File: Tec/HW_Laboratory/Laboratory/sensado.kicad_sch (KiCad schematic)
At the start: 21 parts, among them U5 INA3221, U6 INA3221, U7 LM75B

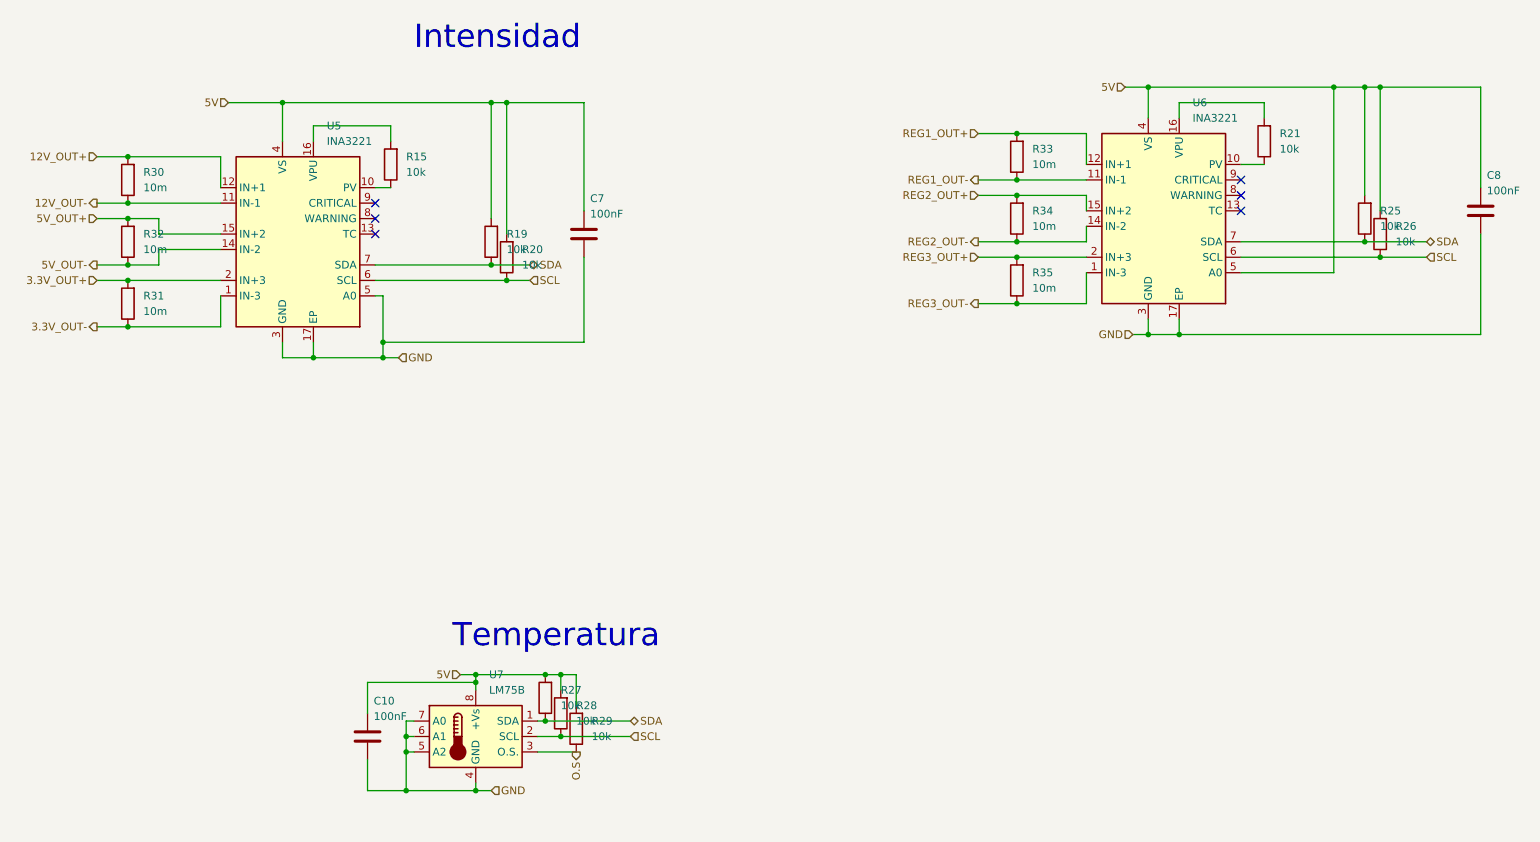
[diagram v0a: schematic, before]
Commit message: Laboratory v2.0:Update the PCB and the Software
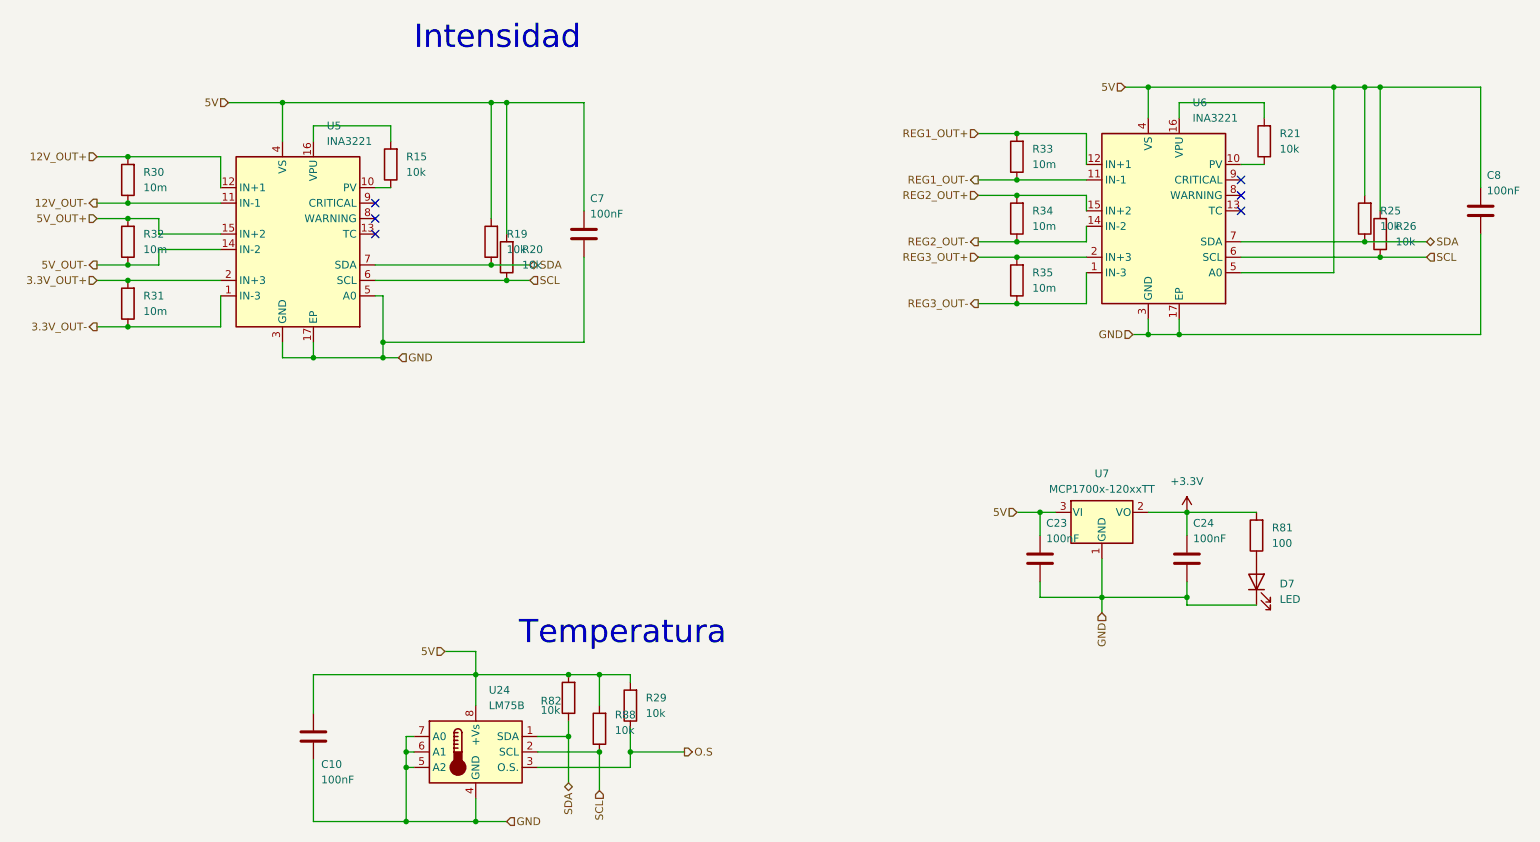
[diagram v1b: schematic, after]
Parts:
- removed R27, R28: 10k, Resistor_SMD:R_0603_1608Metric, symbol Device:R
- removed U7: LM75B, Package_SO:SOIC-8_3.9x4.9mm_P1.27mm, symbol Sensor_Temperature:LM75B
- added C23, C24: 100nF, Capacitor_SMD:C_0603_1608Metric, symbol Device:C
- added D7: LED, LED_SMD:LED_0603_1608Metric, symbol Device:LED
- added R81: 100, Resistor_SMD:R_0603_1608Metric, symbol Device:R
- added R82, R88: 10k, Resistor_SMD:R_0603_1608Metric, symbol Device:R
- added U24: LM75B, Package_SO:SOIC-8_3.9x4.9mm_P1.27mm, symbol Sensor_Temperature:LM75B
- added U7: MCP1700x-120xxTT, Package_TO_SOT_SMD:SOT-23, symbol Regulator_Linear:MCP1700x-120xxTT
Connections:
- net 5V: now also C23.1, R82.2, R88.2, U24.8 (+Vs), U7.3 (VI)
- net GND: now also C23.2, C24.2, D7.1 (K), U24.4 (GND), U24.5 (A2), U24.6 (A1), U24.7 (A0), U7.1 (GND)
- net O.S: now also U24.3 (O.S.)
- net SCL: now also R88.1, U24.2 (SCL)
- net SDA: now also R82.1, U24.1 (SDA)
- new net: D7.2 (A), R81.1
- new net +3.3V: C24.1, R81.2, U7.2 (VO)
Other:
- moved on the sheet: C10, R29
